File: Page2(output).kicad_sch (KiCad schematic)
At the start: 69 parts, among them J4 Screw_Terminal_01x06, U10 LTV-358T, U11 LTV-358T, U12 LTV-358T, U13 LTV-358T, U14 LTV-358T, U15 PCF8574P, U16 PC817, U17 PC817, U18 ULN2003A, U19 PC817, U20 ULN2003A, U21 PC817, U22 ULN2003A, U23 PC817, U24 ULN2003A, U25 PC817, U26 PC817, U27 PC817, U28 PC817, U29 PC817, U30 PC817, U31 PC817, U32 PC817, U33 PC817, U7 PC817, U9 LTV-358T

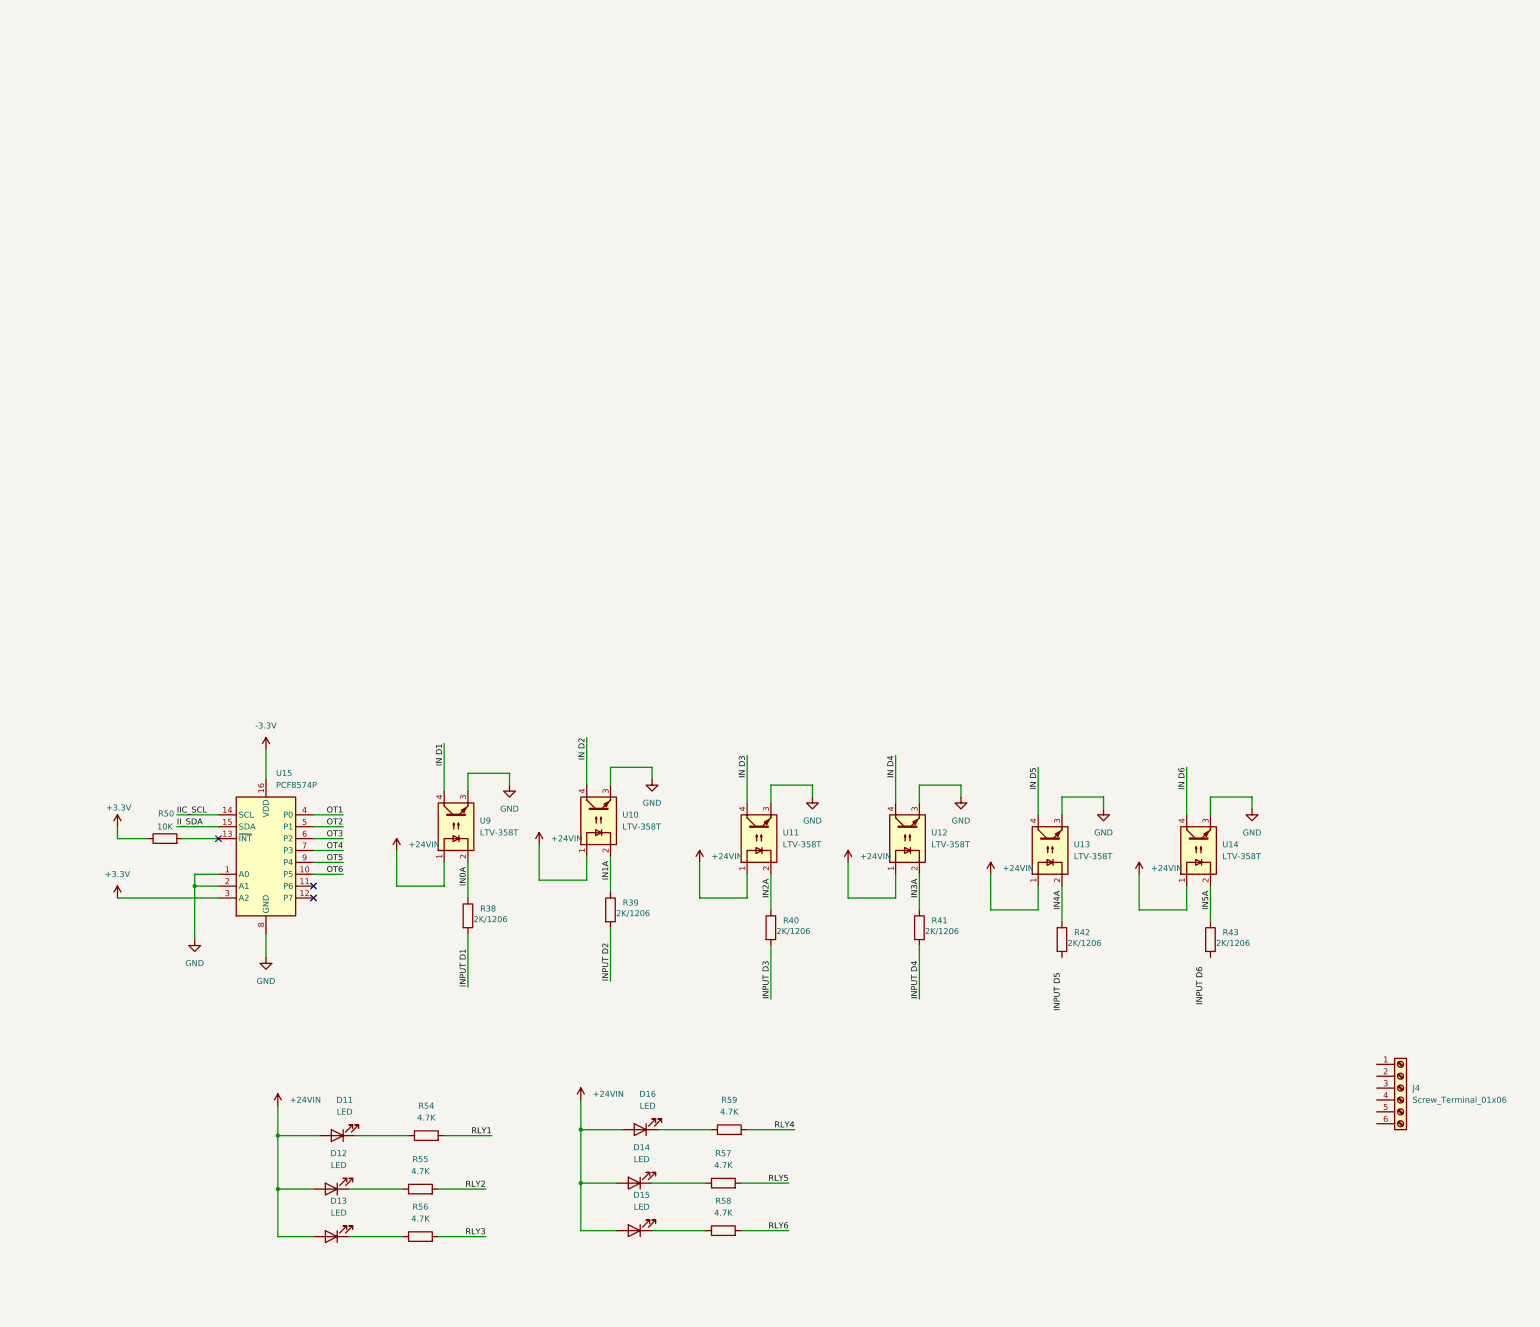
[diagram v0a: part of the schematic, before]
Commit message: :tada: Completing minor touches
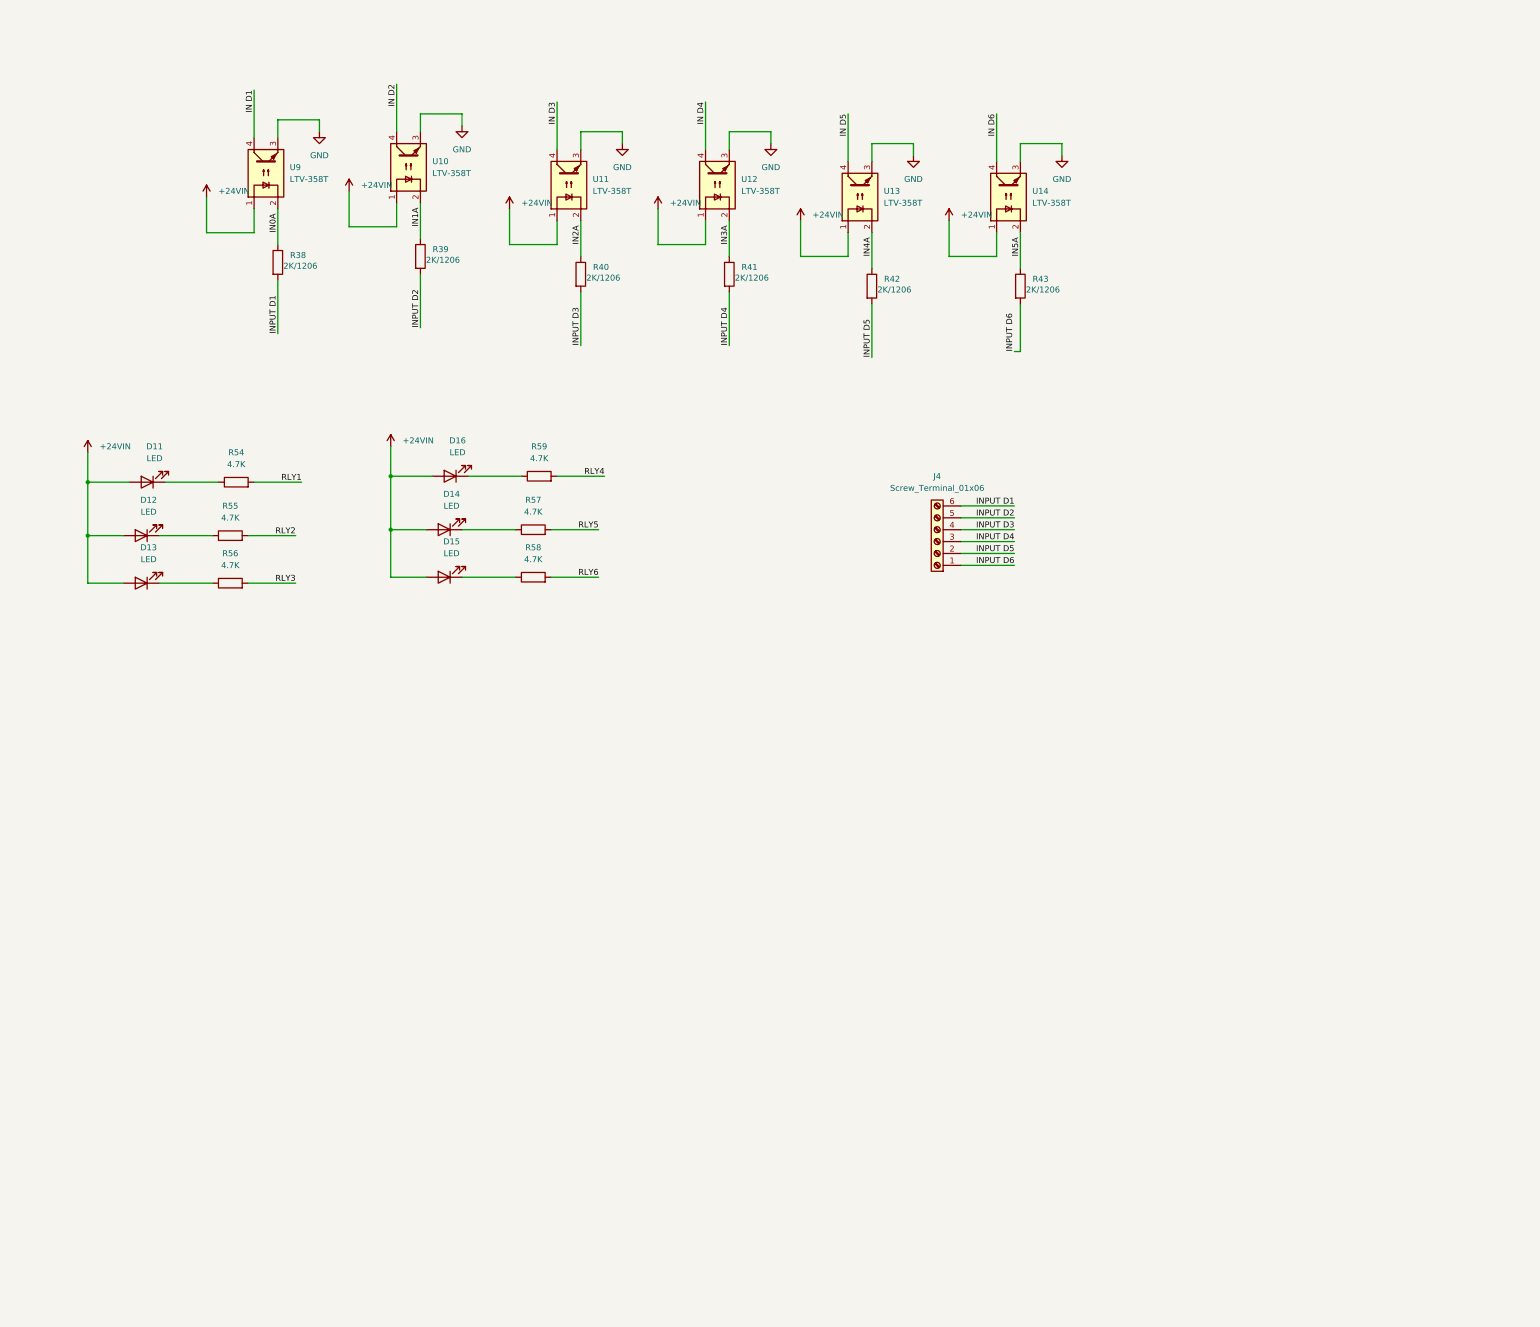
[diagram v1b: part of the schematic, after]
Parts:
- removed R50: 10K, Resistor_THT:R_Axial_DIN0614_L14.3mm_D5.7mm_P5.08mm_Vertical, symbol Device:R
- removed U15: PCF8574P, Package_DIP:DIP-16_W7.62mm, symbol Interface_Expansion:PCF8574P
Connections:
- net INPUT D1: now also J4.6 (Pin_6)
- net INPUT D2: now also J4.5 (Pin_5)
- net INPUT D3: now also J4.4 (Pin_4)
- net INPUT D4: now also J4.3 (Pin_3)
- net INPUT D5: now also J4.2 (Pin_2), R42.2
- net INPUT D6: now also J4.1 (Pin_1), R43.2
- no-connect marks 7 -> 4
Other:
- moved on the sheet: D11, D12, D13, D14, D15, D16, J4, R38, R39, R40, R41, R42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
